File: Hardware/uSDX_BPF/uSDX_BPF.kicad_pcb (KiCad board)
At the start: 2 copper layers, 44.5 x 14 mm, 18 parts, among them P1 GND, P2 GND, P3 ANT2, P4 ANT1, P5 +12V, P6 TX, P7 RX, P8 GND

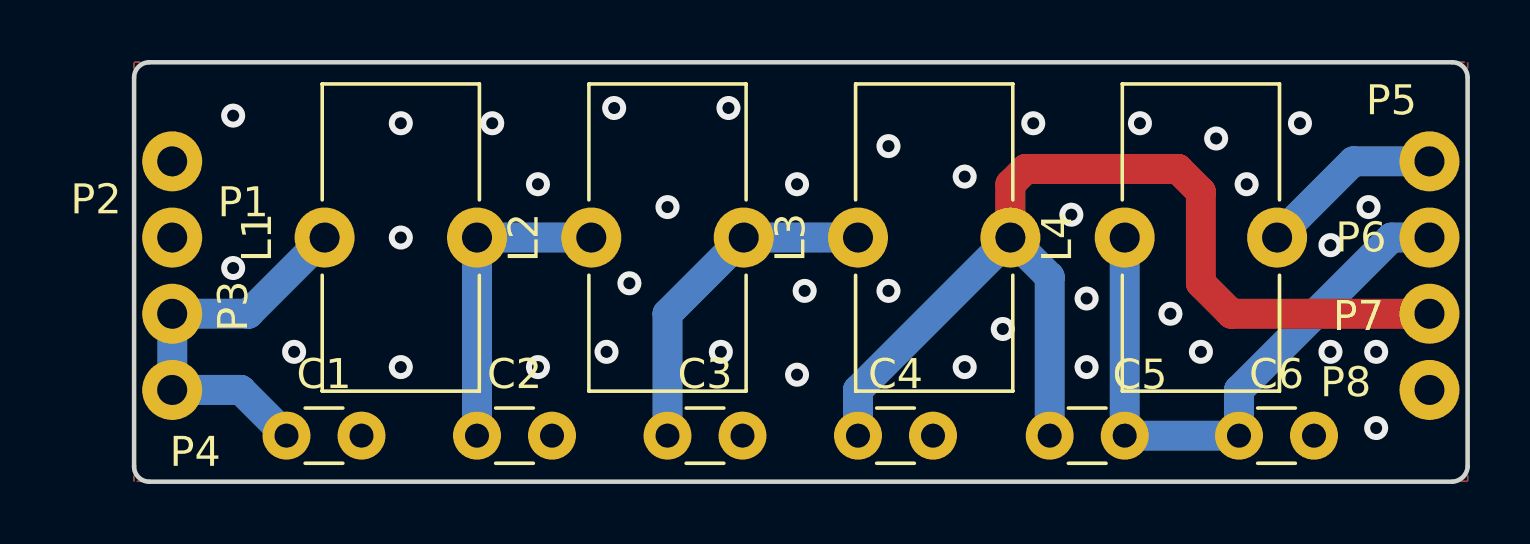
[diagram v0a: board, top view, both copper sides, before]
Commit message: update library locations
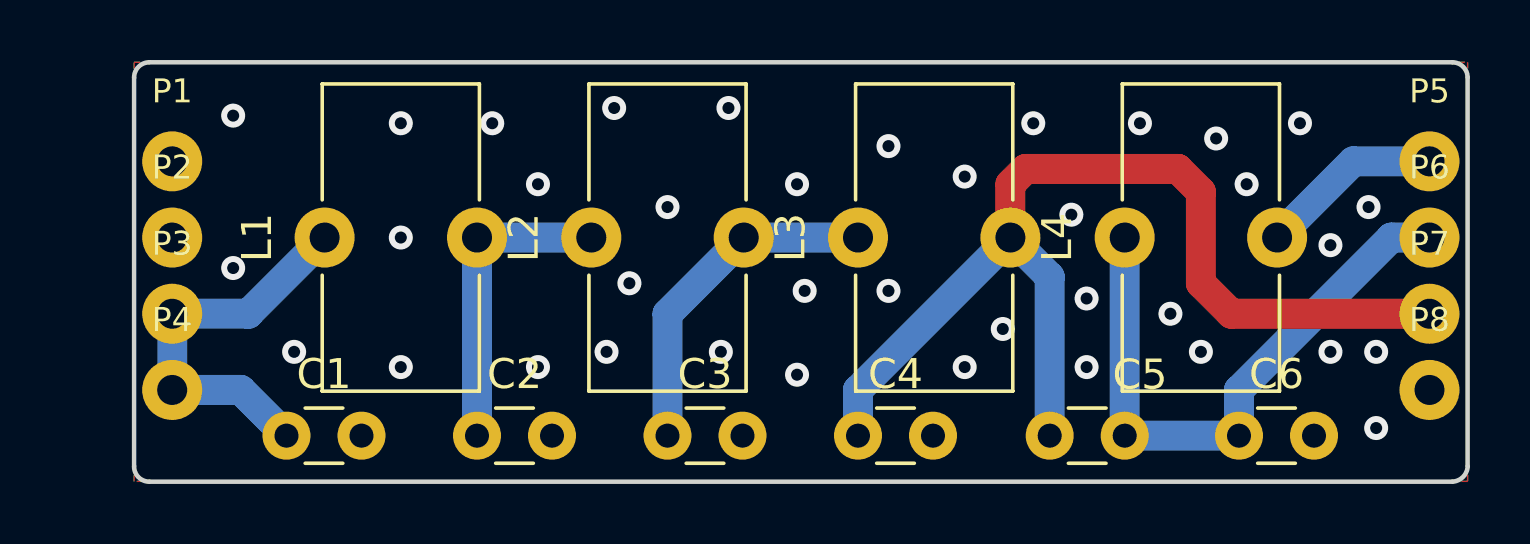
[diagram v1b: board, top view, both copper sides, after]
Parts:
- moved P5 2.70 mm to (97.8, 36.5)
- moved P6 1.10 mm to (97.8, 39.1)
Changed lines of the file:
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@@
   )
   (footprint "user_footprints:pin" (layer "F.Cu")
-    (at 95.09 36.5252)
-    (property "Sheetfile" "uSDX_BPF.kicad_sch")
-    (property "Sheetname" "")
-    (attr through_hole)
-    (fp_text reference "P5" (at 1.43 -2.2352) (layer "F.SilkS")
-      (effects (font (size 1 1) (thickness 0.15)))
-    )
-    (fp_text value "+12V" (at -4.91 -1.3932) (layer "F.Fab")
-      (effects (font (size 1 1) (thickness 0.15)))
-    )
-    (pad "1" thru_hole circle locked (at 2.7 -0.2032) (size 2 2) (drill 1) (layers *.Cu *.Mask)
+    (at 97.79 36.5252)
+    (property "Sheetfile" "uSDX_BPF.kicad_sch")
+    (property "Sheetname" "")
+    (attr through_hole)
+    (fp_text reference "P5" (at 0 -2.54) (layer "F.SilkS")
+      (effects (font (size 0.8 0.8) (thickness 0.1)))
+    )
+    (fp_text value "+12V" (at 0 -5.08) (layer "F.Fab")
+      (effects (font (size 0.8 0.8) (thickness 0.1)))
+    )
+    (pad "1" thru_hole circle (at 0 -0.2032) (size 2 2) (drill 1) (layers *.Cu *.Mask)
       (net 7 "Net-(L4-Pad2)") (pintype "unspecified"))
-    (model "C:/Users/Liviu/Documents/Projects/uSDX_variant/Hardware/3D_models/filterStandoff.step"
-      (offset (xyz 2.7 0 0))
+    (model "${KICAD6_3DMODEL_DIR}/filterStandoff.step"
+      (offset (xyz 0 0 0))
       (scale (xyz 1 1 1))
       (rotate (xyz 0 0 0))
@@
     (property "Sheetname" "")
     (attr through_hole)
-    (fp_text reference "P7" (at -2.37 -0.1232) (layer "F.SilkS")
-      (effects (font (size 1 1) (thickness 0.15)))
-    )
-    (fp_text value "RX" (at -3.64 -0.1232) (layer "F.Fab")
-      (effects (font (size 1 1) (thickness 0.15)))
-    )
-    (pad "1" thru_hole circle locked (at 0 -0.2032) (size 2 2) (drill 1) (layers *.Cu *.Mask)
+    (fp_text reference "P7" (at 0 -2.54) (layer "F.SilkS")
+      (effects (font (size 0.8 0.8) (thickness 0.1)))
+    )
+    (fp_text value "RX" (at 0 -5.08) (layer "F.Fab")
+      (effects (font (size 0.8 0.8) (thickness 0.1)))
+    )
+    (pad "1" thru_hole circle (at 0 -0.2032) (size 2 2) (drill 1) (layers *.Cu *.Mask)
       (net 5 "Net-(C4-Pad1)") (pintype "unspecified"))
-    (model "C:/Users/Liviu/Documents/Projects/uSDX_variant/Hardware/3D_models/filterStandoff.step"
+    (model "${KICAD6_3DMODEL_DIR}/filterStandoff.step"
       (offset (xyz 0 0 0))
       (scale (xyz 1 1 1))
@@
     (property "Sheetname" "")
     (attr through_hole)
-    (fp_text reference "P8" (at -2.794 -0.4572) (layer "F.SilkS")
-      (effects (font (size 1 1) (thickness 0.15)))
-    )
-    (fp_text value "GND" (at -2.37 -0.1232) (layer "F.Fab")
-      (effects (font (size 1 1) (thickness 0.15)))
-    )
-    (pad "1" thru_hole circle locked (at 0 -0.2032) (size 2 2) (drill 1) (layers *.Cu *.Mask)
+    (fp_text reference "P8" (at 0 -2.54) (layer "F.SilkS")
+      (effects (font (size 0.8 0.8) (thickness 0.1)))
+    )
+    (fp_text value "GND" (at 0 -5.08) (layer "F.Fab")
+      (effects (font (size 0.8 0.8) (thickness 0.1)))
+    )
+    (pad "1" thru_hole circle (at 0 -0.2032) (size 2 2) (drill 1) (layers *.Cu *.Mask)
       (net 1 "GND") (pintype "unspecified"))
     (model "${KICAD6_3DMODEL_DIR}/filterStandoff.step"
@@
     (property "Sheetname" "")
     (attr through_hole)
-    (fp_text reference "P4" (at 0.765353 1.864672) (layer "F.SilkS")
-      (effects (font (size 1 1) (thickness 0.15)))
-    )
-    (fp_text value "ANT1" (at -3.81 -0.2032) (layer "F.Fab")
-      (effects (font (size 1 1) (thickness 0.15)))
-    )
-    (pad "1" thru_hole circle locked (at 0 -0.2032) (size 2 2) (drill 1) (layers *.Cu *.Mask)
+    (fp_text reference "P4" (at 0 -2.54) (layer "F.SilkS")
+      (effects (font (size 0.8 0.8) (thickness 0.1)))
+    )
+    (fp_text value "ANT1" (at 0 -5.08) (layer "F.Fab")
+      (effects (font (size 0.8 0.8) (thickness 0.1)))
+    )
+    (pad "1" thru_hole circle (at 0 -0.2032) (size 2 2) (drill 1) (layers *.Cu *.Mask)
       (net 2 "Net-(C1-Pad1)") (pintype "unspecified"))
-    (model "C:/Users/Liviu/Documents/Projects/uSDX_variant/Hardware/3D_models/filterStandoff.step"
+    (model "${KICAD6_3DMODEL_DIR}/filterStandoff.step"
       (offset (xyz 0 0 0))
       (scale (xyz 1 1 1))
@@
     (property "Sheetname" "")
     (attr through_hole)
-    (fp_text reference "P2" (at -2.54 -1.4732) (layer "F.SilkS")
-      (effects (font (size 1 1) (thickness 0.15)))
-    )
-    (fp_text value "GND" (at -2.54 -0.2032) (layer "F.Fab")
-      (effects (font (size 1 1) (thickness 0.15)))
-    )
-    (pad "1" thru_hole circle locked (at 0 -0.2032) (size 2 2) (drill 1) (layers *.Cu *.Mask)
+    (fp_text reference "P2" (at 0 -2.54) (layer "F.SilkS")
+      (effects (font (size 0.8 0.8) (thickness 0.1)))
+    )
+    (fp_text value "GND" (at 0 -5.08) (layer "F.Fab")
+      (effects (font (size 0.8 0.8) (thickness 0.1)))
+    )
+    (pad "1" thru_hole circle (at 0 -0.2032) (size 2 2) (drill 1) (layers *.Cu *.Mask)
       (net 1 "GND") (pintype "unspecified"))
-    (model "C:/Users/Liviu/Documents/Projects/uSDX_variant/Hardware/3D_models/filterStandoff.step"
-      (offset (xyz 0 0 0))
-      (scale (xyz 1 1 1))
-      (rotate (xyz 0 0 0))
-    )
-  )
-  (footprint "user_footprints:pin" (layer "F.Cu")
-    (at 96.69 39.0652)
-    (property "Sheetfile" "uSDX_BPF.kicad_sch")
-    (property "Sheetname" "")
-    (attr through_hole)
-    (fp_text reference "P6" (at -1.186 -0.2032) (layer "F.SilkS")
-      (effects (font (size 1 1) (thickness 0.15)))
-    )
-    (fp_text value "TX" (at -3.64 -0.1232) (layer "F.Fab")
-      (effects (font (size 1 1) (thickness 0.15)))
-    )
-    (pad "1" thru_hole circle locked (at 1.1 -0.2032) (size 2 2) (drill 1) (layers *.Cu *.Mask)
+    (model "${KICAD6_3DMODEL_DIR}/filterStandoff.step"
+      (offset (xyz 0 0 0))
+      (scale (xyz 1 1 1))
+      (rotate (xyz 0 0 0))
+    )
+  )
+  (footprint "user_footprints:pin" (layer "F.Cu")
+    (at 97.79 39.0652)
+    (property "Sheetfile" "uSDX_BPF.kicad_sch")
+    (property "Sheetname" "")
+    (attr through_hole)
+    (fp_text reference "P6" (at 0 -2.54) (layer "F.SilkS")
+      (effects (font (size 0.8 0.8) (thickness 0.1)))
+    )
+    (fp_text value "TX" (at 0 -5.08) (layer "F.Fab")
+      (effects (font (size 0.8 0.8) (thickness 0.1)))
+    )
+    (pad "1" thru_hole circle (at 0 -0.2032) (size 2 2) (drill 1) (layers *.Cu *.Mask)
       (net 6 "Net-(C5-Pad1)") (pintype "unspecified"))
-    (model "C:/Users/Liviu/Documents/Projects/uSDX_variant/Hardware/3D_models/filterStandoff.step"
-      (offset (xyz 1.1 0 0))
+    (model "${KICAD6_3DMODEL_DIR}/filterStandoff.step"
+      (offset (xyz 0 0 0))
       (scale (xyz 1 1 1))
       (rotate (xyz 0 0 0))
@@
     (property "Sheetname" "")
     (attr through_hole)
-    (fp_text reference "P1" (at 2.365346 1.164703 180) (layer "F.SilkS")
-      (effects (font (size 1 1) (thickness 0.15)))
-    )
-    (fp_text value "GND" (at -2.54 -1.4732) (layer "F.Fab")
-      (effects (font (size 1 1) (thickness 0.15)))
-    )
-    (pad "1" thru_hole circle locked (at 0 -0.2032) (size 2 2) (drill 1) (layers *.Cu *.Mask)
+    (fp_text reference "P1" (at 0 -2.54) (layer "F.SilkS")
+      (effects (font (size 0.8 0.8) (thickness 0.1)))
+    )
+    (fp_text value "GND" (at 0 -5.08) (layer "F.Fab")
+      (effects (font (size 0.8 0.8) (thickness 0.1)))
+    )
+    (pad "1" thru_hole circle (at 0 -0.2032) (size 2 2) (drill 1) (layers *.Cu *.Mask)
       (net 1 "GND") (pintype "unspecified"))
-    (model "C:/Users/Liviu/Documents/Projects/uSDX_variant/Hardware/3D_models/filterStandoff.step"
+    (model "${KICAD6_3DMODEL_DIR}/filterStandoff.step"
       (offset (xyz 0 0 0))
       (scale (xyz 1 1 1))
@@
     (property "Sheetname" "")
     (attr through_hole)
-    (fp_text reference "P3" (at 2.032 -0.4572 90) (layer "F.SilkS")
-      (effects (font (size 1 1) (thickness 0.15)))
-    )
-    (fp_text value "ANT2" (at -5.08 -0.2032) (layer "F.Fab")
-      (effects (font (size 1 1) (thickness 0.15)))
-    )
-    (pad "1" thru_hole circle locked (at 0 -0.2032) (size 2 2) (drill 1) (layers *.Cu *.Mask)
+    (fp_text reference "P3" (at 0 -2.54) (layer "F.SilkS")
+      (effects (font (size 0.8 0.8) (thickness 0.1)))
+    )
+    (fp_text value "ANT2" (at 0 -5.08) (layer "F.Fab")
+      (effects (font (size 0.8 0.8) (thickness 0.1)))
+    )
+    (pad "1" thru_hole circle (at 0 -0.2032) (size 2 2) (drill 1) (layers *.Cu *.Mask)
       (net 2 "Net-(C1-Pad1)") (pintype "unspecified"))
-    (model "C:/Users/Liviu/Documents/Projects/uSDX_variant/Hardware/3D_models/filterStandoff.step"
-      (offset (xyz 0 0 0))
-      (scale (xyz 1 1 1))
+    (model "${KICAD6_3DMODEL_DIR}/filterStandoff.step"
+      (offset (xyz 0 0 0))
+      (scale (xyz 1 1 1))
